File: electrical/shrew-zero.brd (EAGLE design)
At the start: 18 x 20 mm, 45 parts, among them IC1 LMR16006YQ3DDCTQ1, U1 ESP32-PICO-D4, U2 SX1280IMLTRT, X1 PIN-1X-BIG, X2 PIN-1X-BIG, Y1 2450FM07D0034001T, Y2 52MHz TCXO

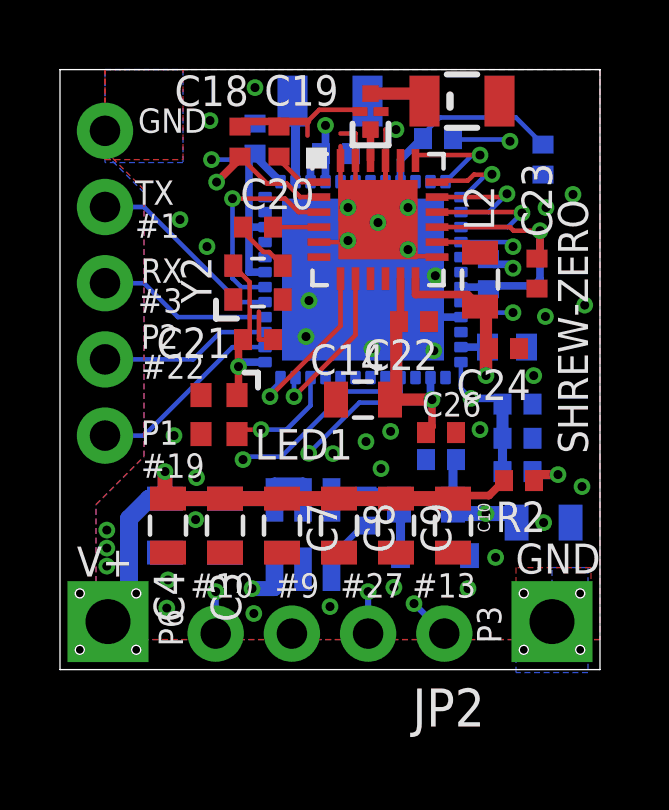
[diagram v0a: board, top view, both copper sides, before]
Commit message: shrew zero next prototype ready to mfg
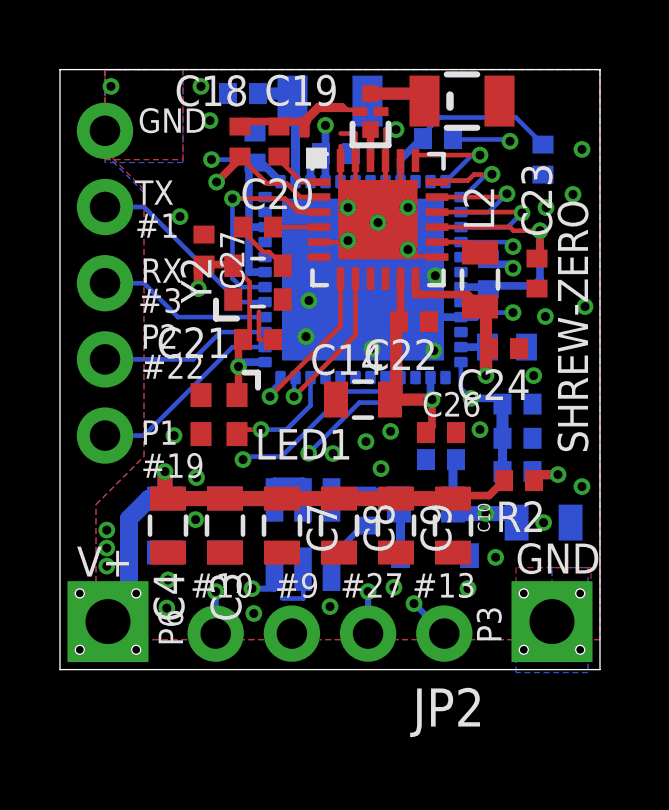
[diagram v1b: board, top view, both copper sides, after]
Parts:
- added C27: 100n, shrew-common:0402-REV
- added C28: 0p5, shrew-common:0402-REV
- ANT1, ANT2: value 74889302450 -> ANT3216LL00R2400A
- moved C11 0.30 mm to (6.50, 17.4)
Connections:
- net 3.3V: now also C27.2
- net GND: now also C27.1, C28.1
- net N$1: now also C28.2
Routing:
- net GND: track 33.7 -> 38.9 mm, vias 39 -> 40
- net 3.3V: track 51.6 -> 53.6 mm, vias 8 -> 9
- net N$1: track 2.78 -> 4.04 mm

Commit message: shrew zero another mfg run
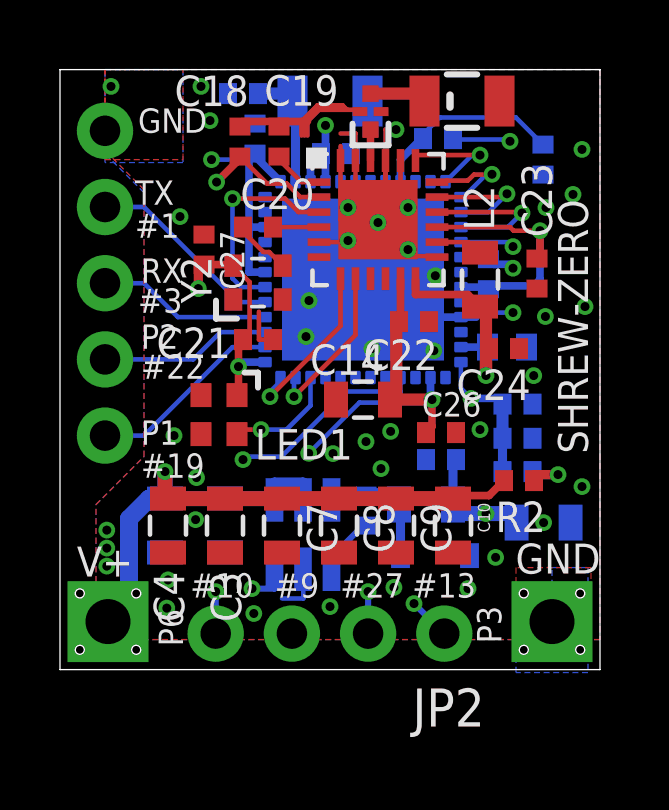
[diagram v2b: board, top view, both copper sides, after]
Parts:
- moved C11 0.30 mm to (6.50, 17.7)
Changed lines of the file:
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@@
 <grid distance="0.1" unitdist="mm" unit="mm" style="dots" multiple="10" display="yes" altdistance="0.01" altunitdist="mm" altunit="mm"/>
 <layers>
-<layer number="1" name="Top" color="4" fill="1" visible="yes" active="yes"/>
+<layer number="1" name="Top" color="4" fill="1" visible="no" active="yes"/>
 <layer number="2" name="Route2" color="1" fill="3" visible="no" active="yes"/>
 <layer number="3" name="Route3" color="4" fill="3" visible="no" active="no"/>
@@
 <layer number="13" name="Route13" color="4" fill="5" visible="no" active="no"/>
 <layer number="14" name="Route14" color="1" fill="6" visible="no" active="no"/>
-<layer number="15" name="Route15" color="4" fill="6" visible="yes" active="yes"/>
+<layer number="15" name="Route15" color="4" fill="6" visible="no" active="yes"/>
 <layer number="16" name="Bottom" color="1" fill="1" visible="yes" active="yes"/>
 <layer number="17" name="Pads" color="2" fill="1" visible="yes" active="yes"/>
@@
 <layer number="21" name="tPlace" color="7" fill="1" visible="yes" active="yes"/>
 <layer number="22" name="bPlace" color="7" fill="1" visible="yes" active="yes"/>
-<layer number="23" name="tOrigins" color="15" fill="1" visible="no" active="yes"/>
-<layer number="24" name="bOrigins" color="15" fill="1" visible="no" active="yes"/>
+<layer number="23" name="tOrigins" color="15" fill="1" visible="yes" active="yes"/>
+<layer number="24" name="bOrigins" color="15" fill="1" visible="yes" active="yes"/>
 <layer number="25" name="tNames" color="7" fill="1" visible="no" active="yes"/>
 <layer number="26" name="bNames" color="7" fill="1" visible="no" active="yes"/>
@@
 <attribute name="VALUE" x="14.1705" y="9.993" size="0.4064" layer="28" rot="MR180"/>
 </element>
-<element name="C11" library="shrew-common" package="0402-REV" value="100n" x="6.5" y="17.4" smashed="yes" rot="MR90">
-<attribute name="NAME" x="7.1985" y="16.511" size="0.4064" layer="26" rot="MR90"/>
-<attribute name="VALUE" x="5.357" y="16.3205" size="0.4064" layer="28" rot="MR90"/>
+<element name="C11" library="shrew-common" package="0402-REV" value="100n" x="6.5" y="17.7" smashed="yes" rot="MR90">
+<attribute name="NAME" x="7.1985" y="16.811" size="0.4064" layer="26" rot="MR90"/>
+<attribute name="VALUE" x="5.357" y="16.6205" size="0.4064" layer="28" rot="MR90"/>
 </element>
 <element name="C15" library="shrew-common" package="0402-REV" value="470n" x="16.1" y="17" smashed="yes" rot="MR90">
@@
 <wire x1="8.85" y1="17.5" x2="8.7" y2="17.2" width="0.254" layer="16"/>
 <wire x1="7.35" y1="16.265" x2="6.565" y2="17.05" width="0.254" layer="16"/>
-<wire x1="6.565" y1="17.05" x2="6.5" y2="16.9" width="0.254" layer="16"/>
+<wire x1="6.565" y1="17.05" x2="6.5" y2="17.2" width="0.254" layer="16"/>
 <wire x1="6.835" y1="14.75" x2="6.3" y2="14.75" width="0.254" layer="16"/>
 <wire x1="6.3" y1="14.75" x2="6.3" y2="17" width="0.254" layer="16"/>
 <wire x1="6.3" y1="17" x2="6.3" y2="17.05" width="0.254" layer="16"/>
-<wire x1="6.3" y1="17.05" x2="6.5" y2="16.9" width="0.254" layer="16"/>
+<wire x1="6.3" y1="17.05" x2="6.5" y2="17.2" width="0.254" layer="16"/>
 <via x="5.05" y="17" extent="1-16" drill="0.3" shape="octagon"/>
 <wire x1="5.05" y1="17" x2="6.3" y2="17" width="0.1524" layer="16"/>
